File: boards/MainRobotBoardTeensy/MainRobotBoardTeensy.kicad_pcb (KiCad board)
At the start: 2 copper layers, 109.6 x 129.9 mm, 108 parts, among them J1 IDC, J10 B3B-XH-A, J11 B3B-XH-A, J12 B3B-XH-A, J13 B3B-XH-A, J14 IDC, J15 IDC, J16 IDC, J2 B3B-XH-A, J3 B3B-XH-A, J4 B3B-XH-A, J5 B3B-XH-A, J6 B3B-XH-A, J7 B3B-XH-A, J8 B3B-XH-A, J9 B3B-XH-A, Q1 MMBT3904LT1G, Q10 MMBT3904LT1G, Q11 MMBT3904LT1G, Q12 MMBT3904LT1G, Q13 MMBT3904LT1G, Q14 MMBT3904LT1G, Q15 MMBT3904LT1G, Q16 MMBT3904LT1G, Q17 MMBT3904LT1G, Q18 MMBT3904LT1G, Q19 MMBT3904LT1G, Q2 MMBT3904LT1G, Q20 MMBT3904LT1G, Q21 MMBT3904LT1G, Q22 MMBT3904LT1G, Q23 MMBT3904LT1G, Q24 MMBT3904LT1G, Q3 MMBT3904LT1G, Q4 MMBT3904LT1G, Q5 MMBT3904LT1G, Q6 MMBT3904LT1G, Q7 MMBT3904LT1G, Q8 MMBT3904LT1G, Q9 MMBT3904LT1G, U1 Teensy4.0, U2 TLC555CDR, U3 SN74HC08DR, U4 SN74HC08DR, U5 PCA9685PW_118, U6 SN74HC08DR, U7 SN74HC08DR, U8 BNO055

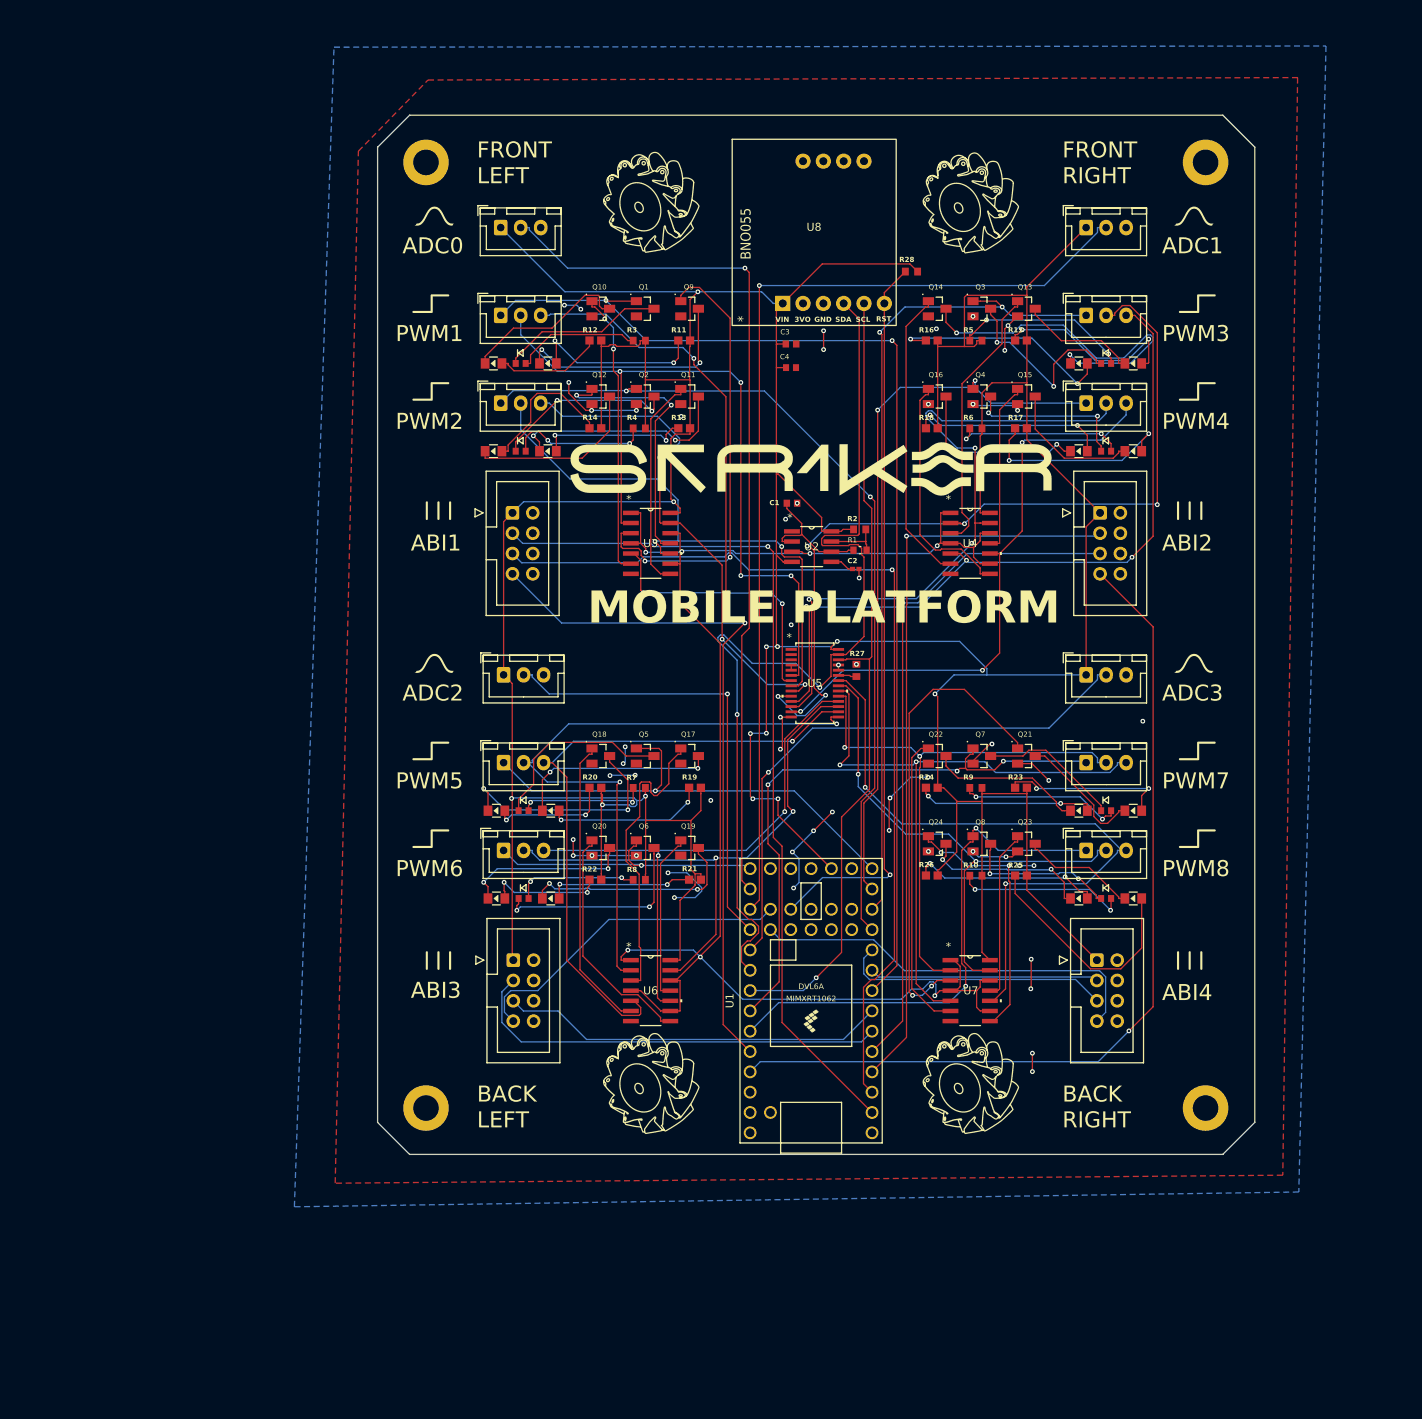
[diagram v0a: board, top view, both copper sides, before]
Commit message: Update main and leg board
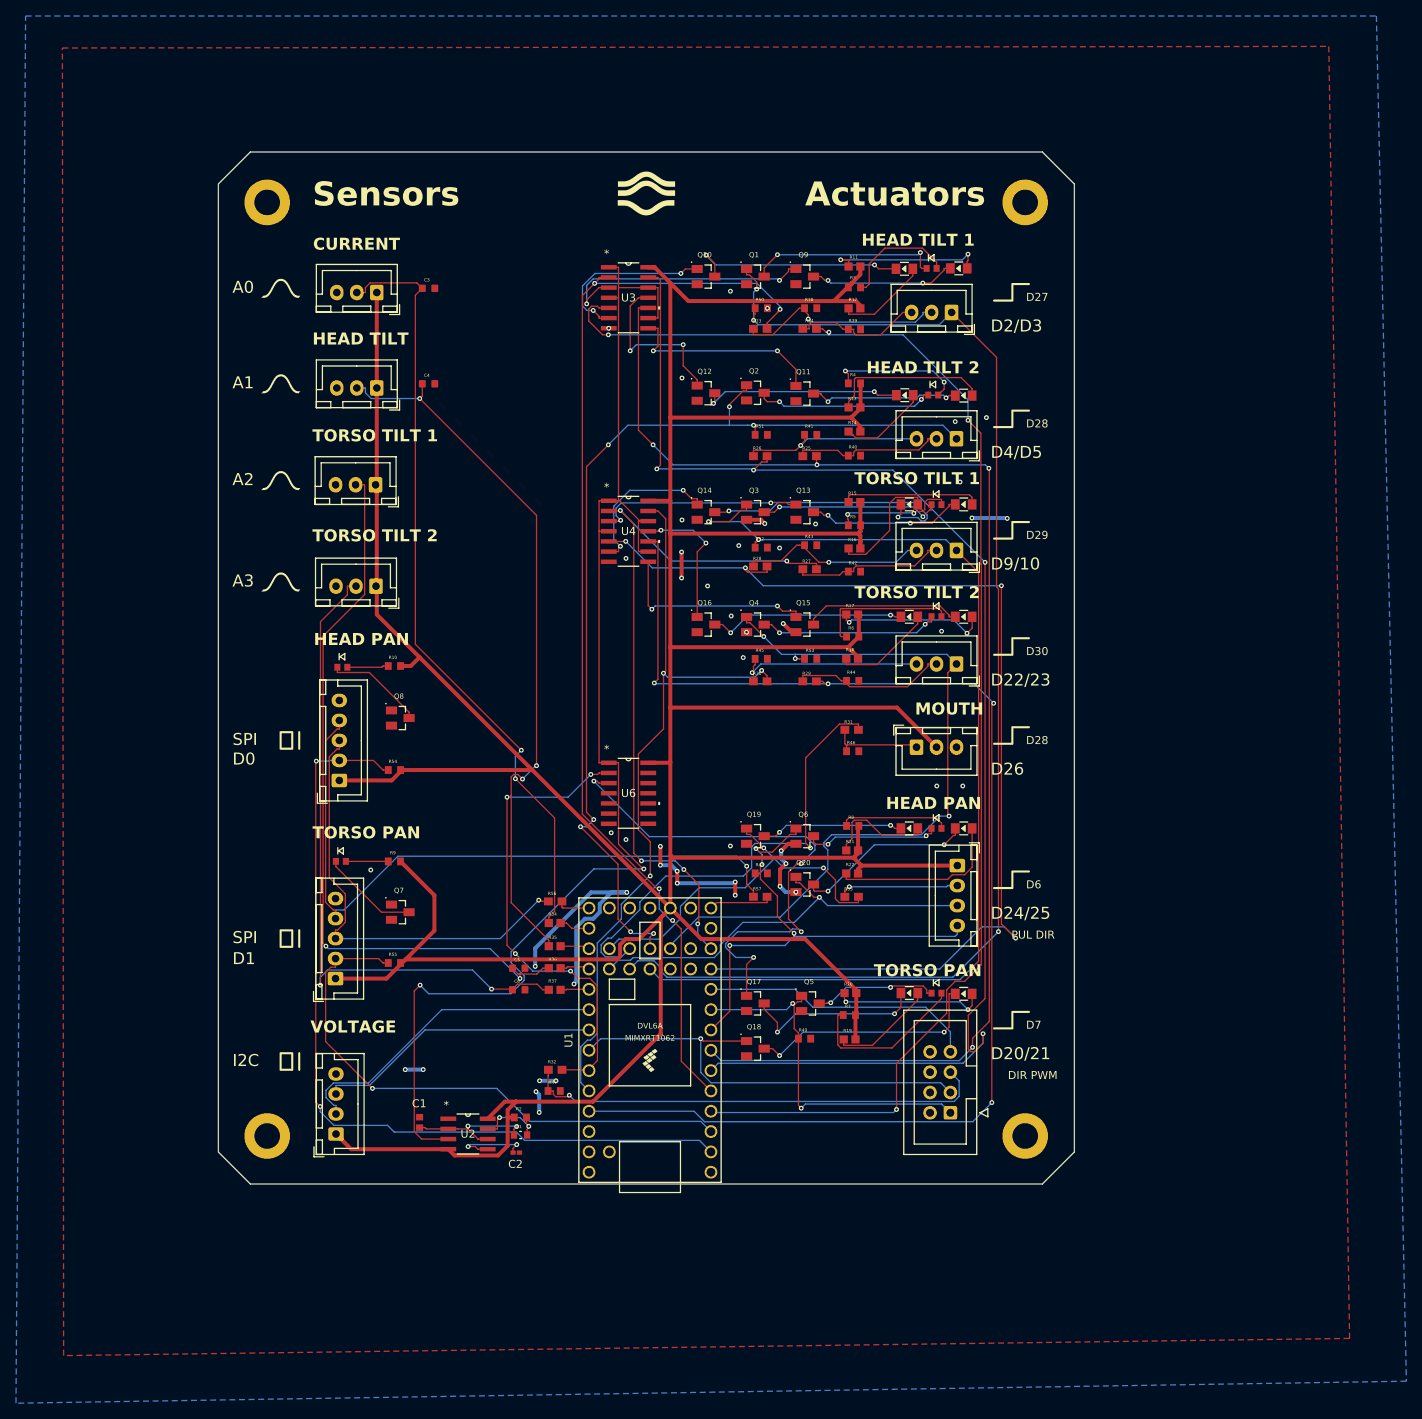
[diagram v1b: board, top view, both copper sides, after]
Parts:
- removed D21, D22, D23, D24: BLUELED, 150080BS75000:150080BS75000_Modified
- removed J15, J16: IDC, Connector_IDC:IDC-Header_2x04_P2.54mm_Vertical
- removed Q21, Q22, Q23, Q24: MMBT3904LT1G, SMMBT3904LT1G:MMBT3904LT1G
- removed U5: PCA9685PW_118, PCA9685PW,118:PCA9685PW,118
- removed U7: SN74HC08DR, SN74HC08DR:SN74HC08DR
- removed U8: BNO055, BNO055:BNO055
- added C5: 47nF, Capacitor47nF:CAPC1608X90N, F.Cu at (110.9, 134.8)
- added C6: 47nF, Capacitor47nF:CAPC1608X90N, F.Cu at (110.9, 137.5)
- added R29: 47R, Resistor47:RESC1608X55, F.Cu at (147.3, 98.9)
- added R30: 47R, Resistor47:RESC1608X55, F.Cu at (141.1, 98.9)
- added R31: 47R, Resistor47:RESC1608X55, F.Cu at (152.6, 105.0)
- added R32: 47R, Resistor47:RESC1608X55, F.Cu at (115.5, 147.5)
- added R33: 47R, Resistor47:RESC1608X55, F.Cu at (152.6, 125.8)
- added R34: 2.2K, Resistor2.2K:RC0603FR-072K2L, F.Cu at (115.4, 129.1)
- added R35: 2.2K, Resistor2.2K:RC0603FR-072K2L, F.Cu at (115.4, 132.0)
- added R36: 2.2K, Resistor2.2K:RC0603FR-072K2L, F.Cu at (115.4, 134.8)
- added R37: 2.2K, Resistor2.2K:RC0603FR-072K2L, F.Cu at (115.4, 137.5)
- added R38: 10K, Resistor10K:CRCW060310K0FKEA, F.Cu at (147.4, 52.3)
- added R39: 10K, Resistor10K:CRCW060310K0FKEA, F.Cu at (152.9, 54.9)
- added R40: 10K, Resistor10K:CRCW060310K0FKEA, F.Cu at (152.9, 70.7)
- added R41: 10K, Resistor10K:CRCW060310K0FKEA, F.Cu at (147.4, 68.1)
- added R42: 10K, Resistor10K:CRCW060310K0FKEA, F.Cu at (152.9, 85.2)
- added R43: 10K, Resistor10K:CRCW060310K0FKEA, F.Cu at (147.4, 81.9)
- added R44: 10K, Resistor10K:CRCW060310K0FKEA, F.Cu at (152.7, 98.9)
- added R45: 10K, Resistor10K:CRCW060310K0FKEA, F.Cu at (141.3, 96.1)
- added R46: 10K, Resistor10K:CRCW060310K0FKEA, F.Cu at (152.7, 107.7)
- added R47: 10K, Resistor10K:CRCW060310K0FKEA, F.Cu at (115.4, 150.1)
- added R48: 10K, Resistor10K:CRCW060310K0FKEA, F.Cu at (141.3, 122.9)
- added R49: 10K, Resistor10K:CRCW060310K0FKEA, F.Cu at (146.7, 143.6)
- added R50: 10K, Resistor10K:CRCW060310K0FKEA, F.Cu at (141.3, 52.3)
- added R51: 10K, Resistor10K:CRCW060310K0FKEA, F.Cu at (141.3, 68.1)
- added R52: 10K, Resistor10K:CRCW060310K0FKEA, F.Cu at (141.3, 82.2)
- added R53: 10K, Resistor10K:CRCW060310K0FKEA, F.Cu at (147.4, 96.1)
- added R54: 10K, Resistor10K:CRCW060310K0FKEA, F.Cu at (95.4, 110.0)
- added R55: 10K, Resistor10K:CRCW060310K0FKEA, F.Cu at (95.4, 134.1)
- added R56: 47R, Resistor47:RESC1608X55, F.Cu at (115.5, 126.4)
- added R57: 47R, Resistor47:RESC1608X55, F.Cu at (141.1, 125.8)
- C1: footprint CC0603JRX7R7BB105:CC0603JRX7R7BB105 -> Capacitor1uF:CC0603JRX7R7BB105
- C2: footprint C0402C103J4RACTU:C0402C103J4RACTU -> Capacitor0.01uF:C0402C103J4RACTU
- C3: value 1uF -> 47nF; footprint CC0603JRX7R7BB105:CC0603JRX7R7BB105 -> Capacitor47nF:CAPC1608X90N
- C4: value 100nF -> 47nF; footprint CC0603KRX7R9BB104:CC0603KRX7R9BB104 -> Capacitor47nF:CAPC1608X90N
- D1, D2, D3, D4, D5, D6, D7, D8: footprint NCD0603R1:NCD0603R1 -> LedRed:NCD0603R1
- D10, D11, D12, D13, D14, D15, D16, D17, D18, D19, D20, D9: footprint 150080BS75000:150080BS75000_Modified -> LedBlue:150080BS75000_Modified
- J1: value IDC -> B3B-XH-A; footprint Connector_IDC:IDC-Header_2x04_P2.54mm_Vertical -> Connector_JST:JST_XH_B3B-XH-A_1x03_P2.50mm_Vertical
- J10, J12: value B3B-XH-A -> B4B-XH-A; footprint Connector_JST:JST_XH_B3B-XH-A_1x03_P2.50mm_Vertical -> Connector_JST:JST_XH_B4B-XH-A_1x04_P2.50mm_Vertical
- J11: value B3B-XH-A -> IDC; footprint Connector_JST:JST_XH_B3B-XH-A_1x03_P2.50mm_Vertical -> Connector_IDC:IDC-Header_2x04_P2.54mm_Vertical
- J13: value B3B-XH-A -> B5B-XH-A; footprint Connector_JST:JST_XH_B3B-XH-A_1x03_P2.50mm_Vertical -> Connector_JST:JST_XH_B5B-XH-A_1x05_P2.50mm_Vertical
- J14: value IDC -> B5B-XH-A; footprint Connector_IDC:IDC-Header_2x04_P2.54mm_Vertical -> Connector_JST:JST_XH_B5B-XH-A_1x05_P2.50mm_Vertical
- Q1, Q10, Q11, Q12, Q13, Q14, Q15, Q16, Q17, Q18, Q19, Q2, Q20, Q3, Q4, Q5, Q6, Q7, Q8, Q9: footprint SMMBT3904LT1G:MMBT3904LT1G -> Transistor:MMBT3904LT1G
- R1: footprint RC0603FR-07360KL:RC0603FR-07360KL -> Resistor360K:RC0603FR-07360KL
- R10, R3, R4, R5, R6, R7, R8, R9: footprint RCG06031K00FKEA:RCG06031K00FKEA -> Resistor1K:RCG06031K00FKEA
- R11, R12, R13, R14, R15, R16, R17, R18, R19, R20, R21, R22: footprint RC0603FR-07150RL:RESC1607X60N -> Resistor150:RESC1607X60N
- R2: footprint CRCW060310K0FKEA:CRCW060310K0FKEA -> Resistor10K:CRCW060310K0FKEA
- R23, R24, R25, R26: value 150R -> 47R; footprint RC0603FR-07150RL:RESC1607X60N -> Resistor47:RESC1608X55
- R27, R28: value 10K -> 47R; footprint CRCW060310K0FKEA:CRCW060310K0FKEA -> Resistor47:RESC1608X55
- U1: footprint Teensy40:Teensy40 -> Teensy:Teensy40
- U2: footprint TLC555CDR:TLC555CDR -> 555Timer:TLC555CDR
- U3, U4, U6: footprint SN74HC08DR:SN74HC08DR -> Gate:SN74HC08DR
- moved J14 111.9 mm to (88.0, 136.1), turned to 90 degrees
- moved J12 104.6 mm to (88.1, 155.5), turned to 90 degrees
- moved D8 99.7 mm to (88.9, 97.2)
- moved D7 95.9 mm to (88.7, 121.4)
- moved J3 94.5 mm to (93.0, 74.3), turned to 180 degrees
- moved J13 93.8 mm to (88.5, 111.3), turned to 90 degrees
- moved C1 90.3 mm to (98.5, 154.1), turned to 90 degrees
- moved U2 85.1 mm to (104.6, 155.5)
- moved R2 84.9 mm to (111.1, 153.4)
- moved R1 84.5 mm to (111.2, 155.6)
- moved C2 84.4 mm to (110.6, 157.8)
- moved R10 77.3 mm to (95.4, 97.0)
- moved Q7 75.3 mm to (96.1, 127.8)
- moved Q8 74.4 mm to (96.1, 103.5)
- moved R9 73.3 mm to (95.4, 121.4)
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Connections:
- net LPWM1BLINK renamed HEADTILT1LPWMBLINK
- net LPWM2BLINK renamed HEADTILT2LPWMBLINK
- net LPWM3BLINK renamed TORSOTILT1LPWMBLINK
- net RPWM1BLINK renamed HEADTILT1RPWMBLINK
- net RPWM2BLINK renamed HEADTILT2RPWMBLINK
- net RPWM3BLINK renamed TORSOTILT1RPWMBLINK
- net RPWM5BLINK renamed TORSOPANPWMBLINK
- C3 pad 1: +3.3V -> Net-(J1-Pin_2)
- C4 pad 1: +3.3V -> Net-(J2-Pin_2)
- J1 pad 2: GND -> Net-(J1-Pin_2)
- J1 pad 3: ENCODER1_A -> GND
- J10 pad 1: PWMEN5 -> +3.3V
- J10 pad 2: RPWM5 -> Net-(J10-Pin_2)
- J10 pad 3: LPWM5 -> HEADPANDIR
- J11 pad 1: PWMEN6 -> TORSOPANEN
- J11 pad 2: RPWM6 -> GND
- J11 pad 3: LPWM6 -> TORSOPANDIR
- J12 pad 1: PWMEN7 -> +3.3V
- J12 pad 2: RPWM7 -> SDA
- J12 pad 3: LPWM7 -> SCL
- J13 pad 1: PWMEN8 -> +3.3V
- J13 pad 2: RPWM8 -> CSHEAD
- J13 pad 3: LPWM8 -> SCK
- J14 pad 2: GND -> CSTORSO
- J14 pad 3: ENCODER2_A -> SCK
- J14 pad 4: GND -> MISO
- J14 pad 5: ENCODER2_B -> GND
- J2 pad 2: A0 -> Net-(J2-Pin_2)
- J3 pad 2: A1 -> Net-(J3-Pin_2)
- J4 pad 2: A2 -> Net-(J4-Pin_2)
- J5 pad 1: +3.3V -> HEADTILT1EN
- J5 pad 2: A3 -> Net-(J5-Pin_2)
- J5 pad 3: GND -> Net-(J5-Pin_3)
- J6 pad 1: PWMEN1 -> HEADTILT2EN
- J6 pad 2: RPWM1 -> Net-(J6-Pin_2)
- J6 pad 3: LPWM1 -> Net-(J6-Pin_3)
- J7 pad 1: PWMEN2 -> TORSOTILT1EN
- J7 pad 2: RPWM2 -> Net-(J7-Pin_2)
- J7 pad 3: LPWM2 -> Net-(J7-Pin_3)
- J8 pad 1: PWMEN3 -> TORSOTILT2EN
- J8 pad 2: RPWM3 -> Net-(J8-Pin_2)
- J8 pad 3: LPWM3 -> Net-(J8-Pin_3)
- J9 pad 1: PWMEN4 -> Net-(J9-Pin_1)
- J9 pad 2: RPWM4 -> +3.3V
- J9 pad 3: LPWM4 -> GND
- Q1 pad 1: PWMEN1 -> HEADTILT1EN
- Q15 pad 1: RPWM4BLINK -> TORSOTILT2RPWMBLINK
- Q16 pad 1: LPWM4BLINK -> TORSOTILT2LPWMBLINK
- Q18 pad 1: LPWM5BLINK -> TORSOPANDIR
- Q19 pad 1: RPWM6BLINK -> HEADPANPUL
- Q2 pad 1: PWMEN2 -> HEADTILT2EN
- Q20 pad 1: LPWM6BLINK -> HEADPANDIR
- Q3 pad 1: PWMEN3 -> TORSOTILT1EN
- Q4 pad 1: PWMEN4 -> TORSOTILT2EN
- Q5 pad 1: PWMEN5 -> TORSOPANEN
- Q6 pad 1: PWMEN6 -> HEADPANEN
- Q7 pad 1: PWMEN7 -> TORSOENCODERST
- Q8 pad 1: PWMEN8 -> HEADENCODERST
- R23 pad 1: Net-(D21-A) -> Net-(J5-Pin_2)
- R23 pad 2: +3.3V -> HEADTILT1RPWM
- R24 pad 1: Net-(D22-A) -> Net-(J5-Pin_3)
- R24 pad 2: +3.3V -> HEADTILT1LPWM
- R25 pad 1: Net-(D23-A) -> Net-(J6-Pin_2)
- R25 pad 2: +3.3V -> HEADTILT2RPWM
- R26 pad 1: Net-(D24-A) -> Net-(J6-Pin_3)
- R26 pad 2: +3.3V -> HEADTILT2LPWM
- R27 pad 1: Net-(U5-*OE) -> Net-(J7-Pin_2)
- R27 pad 2: GND -> TORSOTILT1RPWM
- R28 pad 1: RST -> Net-(J7-Pin_3)
- R28 pad 2: +3.3V -> TORSOTILT1LPWM
- U1 pad 10: ENCODER4_B -> TORSOPANST
- U1 pad 11: PWMEN2 -> TORSOTILT1LPWM
- U1 pad 12: PWMEN3 -> TORSOTILT1RPWM
- U1 pad 13: PWMEN4 -> unconnected-(U1-11_MOSI_CTX1-Pad13)
- U1 pad 14: PWMEN5 -> Net-(U1-12_MISO_MQSL)
- U1 pad 2: ENCODER1_A -> CSHEAD
- U1 pad 20: PWMEN6 -> Net-(U1-13_SCK_CRX1_LED)
- U1 pad 21: A0 -> CURRENT
- U1 pad 22: A1 -> HEAD
- U1 pad 23: A2 -> TORSO1
- U1 pad 24: A3 -> TORSO2
- U1 pad 27: PWMEN7 -> TORSOPANDIR
- U1 pad 28: PWMEN8 -> TORSOPANPWM
- U1 pad 29: ENCODER1_I -> TORSOTILT2LPWM
- U1 pad 3: ENCODER1_B -> CSTORSO
- U1 pad 30: ENCODER2_I -> TORSOTILT2RPWM
- U1 pad 35: ENCODER3_I -> HEADPANPUL
- U1 pad 36: ENCODER4_I -> HEADPANDIR
- U1 pad 37: RST -> MOUTHSERVO
- U1 pad 38: unconnected-(U1-27_A13_SCK1-Pad38) -> HEADTILT1EN
- U1 pad 39: unconnected-(U1-28_RX7-Pad39) -> HEADTILT2EN
- U1 pad 4: ENCODER2_A -> HEADTILT1LPWM
- U1 pad 40: unconnected-(U1-29_TX7-Pad40) -> TORSOTILT1EN
- U1 pad 41: unconnected-(U1-30_CRX3-Pad41) -> TORSOTILT2EN
- U1 pad 5: ENCODER2_B -> HEADTILT1RPWM
- U1 pad 6: ENCODER3_A -> HEADTILT2LPWM
- U1 pad 7: ENCODER3_B -> HEADTILT2RPWM
- U1 pad 8: PWMEN1 -> HEADPANEN
- U1 pad 9: ENCODER4_A -> TORSOPANEN
- U3 pad 10: RPWM2 -> HEADTILT2RPWM
- U3 pad 13: LPWM2 -> HEADTILT2LPWM
- U3 pad 2: RPWM1 -> HEADTILT1RPWM
- U3 pad 5: LPWM1 -> HEADTILT1LPWM
- U4 pad 10: LPWM4 -> TORSOTILT2RPWM
- U4 pad 11: RPWM4BLINK -> TORSOTILT2LPWMBLINK
- U4 pad 13: RPWM4 -> TORSOTILT2LPWM
- U4 pad 2: RPWM3 -> TORSOTILT1RPWM
- U4 pad 5: LPWM3 -> TORSOTILT1LPWM
- U4 pad 8: LPWM4BLINK -> TORSOTILT2RPWMBLINK
- U6 pad 10: LPWM6 -> unconnected-(U6-3B-Pad10)
- U6 pad 11: RPWM6BLINK -> unconnected-(U6-4Y-Pad11)
- U6 pad 12: BLINK -> unconnected-(U6-4A-Pad12)
- U6 pad 13: RPWM6 -> unconnected-(U6-4B-Pad13)
- U6 pad 2: RPWM5 -> TORSOPANPWM
- U6 pad 4: BLINK -> unconnected-(U6-2A-Pad4)
- U6 pad 5: LPWM5 -> unconnected-(U6-2B-Pad5)
- U6 pad 6: LPWM5BLINK -> unconnected-(U6-2Y-Pad6)
- U6 pad 8: LPWM6BLINK -> unconnected-(U6-3Y-Pad8)
- U6 pad 9: BLINK -> unconnected-(U6-3A-Pad9)
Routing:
- net HEADTILT2LPWM: track 0.00 -> 176.1 mm, vias 0 -> 4
- net HEADTILT1LPWM: track 0.00 -> 175.7 mm, vias 0 -> 4
- net HEADTILT2RPWM: track 0.00 -> 170.6 mm, vias 0 -> 4
- net TORSOTILT2RPWM: track 0.00 -> 166.1 mm, vias 0 -> 4
- net HEADTILT1EN: track 0.00 -> 164.3 mm, vias 0 -> 3
- net TORSOTILT1LPWM: track 0.00 -> 140.8 mm, vias 0 -> 4
- net HEADTILT1RPWM: track 0.00 -> 138.6 mm, vias 0 -> 4
- net PWMEN1: track 138.4 -> 0.00 mm, vias 2 -> 0
- net TORSOTILT1EN: track 0.00 -> 134.9 mm, vias 0 -> 3
- net A1: track 125.1 -> 0.00 mm, vias 1 -> 0
- net HEADTILT2EN: track 0.00 -> 123.8 mm, vias 0 -> 7
- net ENCODER1_B: track 117.0 -> 0.00 mm, vias 1 -> 0
- net ENCODER2_I: track 110.6 -> 0.00 mm, vias 1 -> 0
- net PWMEN2: track 109.3 -> 0.00 mm, vias 2 -> 0
- net A0: track 108.9 -> 0.00 mm, vias 1 -> 0
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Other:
- board size 109.6 x 129.9 mm -> 107 x 129 mm
- board text added: "A0"
- board text added: "A1"
- board text added: "A2"
- board text added: "A3"
- board text added: "Actuators"
- board text added: "CURRENT"
- board text added: "D0"
- board text added: "D1"
- board text added: "D2/D3"
- board text added: "D20/21"
- board text added: "D22/23"
- board text added: "D24/25"
- board text added: "D26"
- board text added: "D27"
- board text added: "D28"
- board text added: "D29"
- board text added: "D30"
- board text added: "D4/D5"
- board text added: "D6"
- board text added: "D7"
- board text added: "D9/10"
- board text added: "DIR PWM"
- board text added: "HEAD PAN"
- board text added: "HEAD TILT"
- board text added: "HEAD TILT 1"
- board text added: "HEAD TILT 2"
- board text added: "I2C"
- board text added: "MOUTH"
- board text added: "PUL DIR"
- board text added: "SPI"
- board text added: "Sensors"
- board text added: "TORSO PAN"
- board text added: "TORSO TILT 1"
- board text added: "TORSO TILT 2"
- board text added: "VOLTAGE"
- board text removed: "ABI1"
- board text removed: "ABI2"
- board text removed: "ABI3"
- board text removed: "ABI4"
- board text removed: "ADC0"
- board text removed: "ADC1"
- board text removed: "ADC2"
- board text removed: "ADC3"
- board text removed: "BACK LEFT"
- board text removed: "BACK RIGHT"
- board text removed: "FRONT LEFT"
- board text removed: "FRONT RIGHT"
- board text removed: "MOBILE PLATFORM"
- board text removed: "PWM1"
- board text removed: "PWM2"
- board text removed: "PWM3"
- board text removed: "PWM4"
- board text removed: "PWM5"
- board text removed: "PWM6"
- board text removed: "PWM7"
- board text removed: "PWM8"
